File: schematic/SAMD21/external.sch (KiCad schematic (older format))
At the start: 19 parts, among them IC3 MCP2221-I_SL, J10 Conn_02x06_Odd_Even, J11 Conn_02x06_Odd_Even, J12 Conn_02x06_Odd_Even, J13 Conn_01x02, J14 Conn_02x05_Odd_Even, J15 Conn_01x08, J8 Conn_02x02_Odd_Even, J9 Conn_02x02_Odd_Even

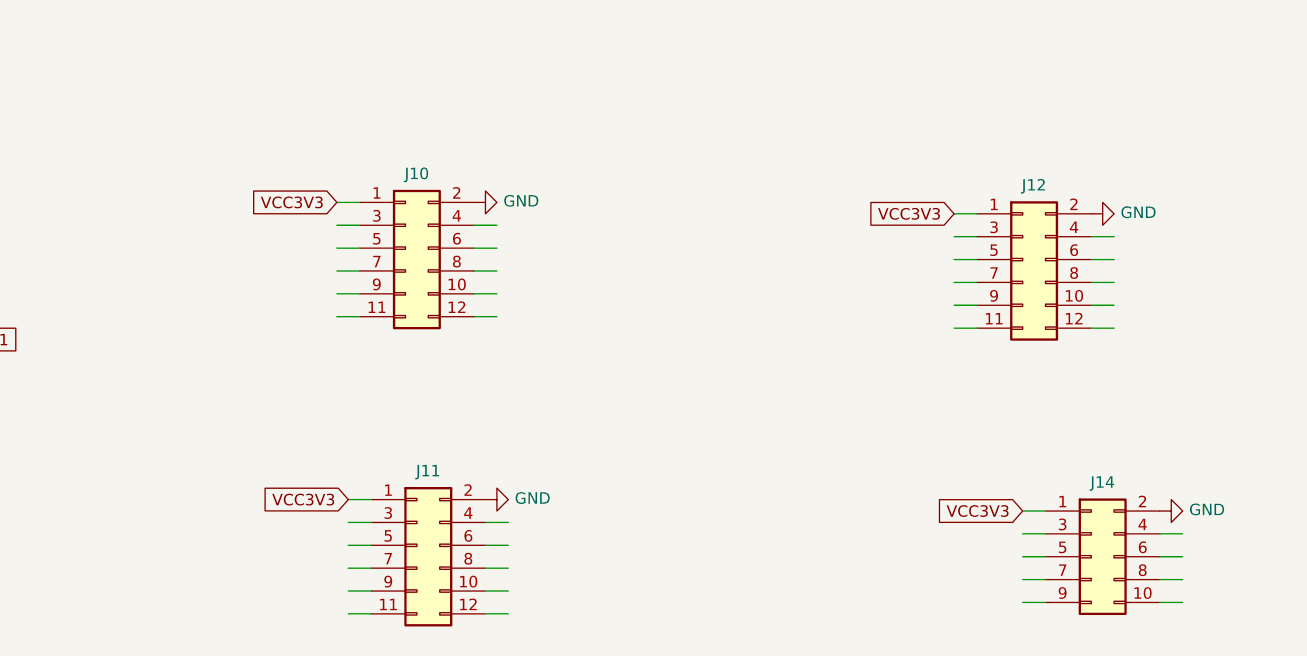
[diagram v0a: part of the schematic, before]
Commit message: Complete schematic
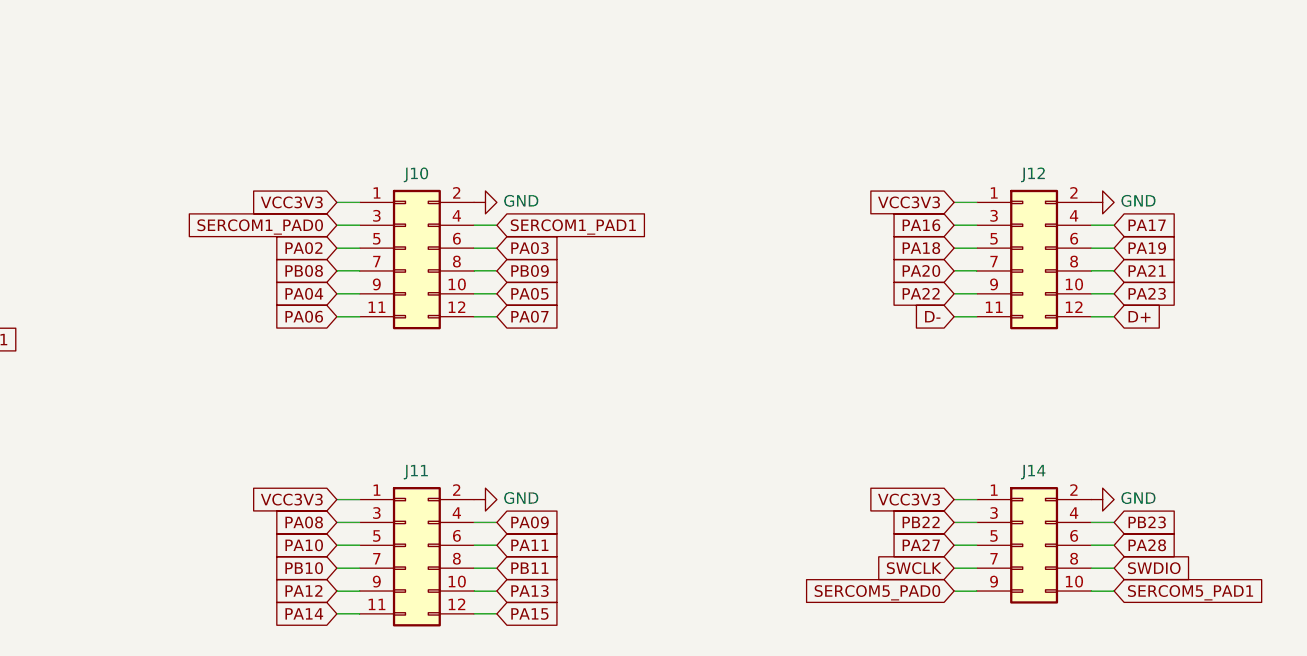
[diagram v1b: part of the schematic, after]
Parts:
- J10: footprint (none) -> Connector_PinHeader_2.54mm:PinHeader_2x06_P2.54mm_Vertical
- J12: footprint (none) -> Connector_PinHeader_2.54mm:PinHeader_2x06_P2.54mm_Vertical_SMD
- J14: footprint (none) -> Connector_PinHeader_2.54mm:PinHeader_2x05_P2.54mm_Vertical
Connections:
- net labels added: D+, D-, PA02, PA03, PA04, PA05, PA06, PA07, PA08, PA09, PA10, PA11, PA12, PA13, PA14, PA15, PA16, PA17, PA18, PA19, PA20, PA21, PA22, PA23, PA27, PA28, PB08, PB09, PB10, PB11, PB22, PB23
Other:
- moved on the sheet: J11, J12, J14
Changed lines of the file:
@@
 L Connector_Generic:Conn_02x06_Odd_Even J11
 U 1 1 61799C22
-P 4850 5800
-F 0 "J11" H 4900 6125 50  0000 C CNN
-F 1 "Conn_02x06_Odd_Even" H 4900 6126 50  0001 C CNN
-F 2 "Connector_PinHeader_2.54mm:PinHeader_2x06_P2.54mm_Vertical" H 4850 5800 50  0001 C CNN
-F 3 "~" H 4850 5800 50  0001 C CNN
-	1    4850 5800
-	1    0    0    -1
-$EndComp
-Text GLabel 7200 4350 0    50   Input ~ 0
-VCC3V3
-Text GLabel 4550 5600 0    50   Input ~ 0
-VCC3V3
-Text GLabel 7500 5650 0    50   Input ~ 0
+P 4800 5800
+F 0 "J11" H 4850 6125 50  0000 C CNN
+F 1 "Conn_02x06_Odd_Even" H 4850 6126 50  0001 C CNN
+F 2 "Connector_PinHeader_2.54mm:PinHeader_2x06_P2.54mm_Vertical" H 4800 5800 50  0001 C CNN
+F 3 "~" H 4800 5800 50  0001 C CNN
+	1    4800 5800
+	1    0    0    -1
+$EndComp
+Text GLabel 7200 4300 0    50   Input ~ 0
+VCC3V3
+Text GLabel 4500 5600 0    50   Input ~ 0
+VCC3V3
+Text GLabel 7200 5600 0    50   Input ~ 0
 VCC3V3
 $Comp
 L power:GND #PWR029
 U 1 1 617AC5C9
-P 7800 4350
-F 0 "#PWR029" H 7800 4100 50  0001 C CNN
-F 1 "GND" V 7805 4222 50  0000 R CNN
-F 2 "" H 7800 4350 50  0001 C CNN
-F 3 "" H 7800 4350 50  0001 C CNN
-	1    7800 4350
+P 7800 4300
+F 0 "#PWR029" H 7800 4050 50  0001 C CNN
+F 1 "GND" V 7805 4172 50  0000 R CNN
+F 2 "" H 7800 4300 50  0001 C CNN
+F 3 "" H 7800 4300 50  0001 C CNN
+	1    7800 4300
 	0    -1   -1   0
 $EndComp
@@
 L power:GND #PWR027
 U 1 1 617B03D0
-P 5150 5600
-F 0 "#PWR027" H 5150 5350 50  0001 C CNN
-F 1 "GND" V 5155 5472 50  0000 R CNN
-F 2 "" H 5150 5600 50  0001 C CNN
-F 3 "" H 5150 5600 50  0001 C CNN
-	1    5150 5600
+P 5100 5600
+F 0 "#PWR027" H 5100 5350 50  0001 C CNN
+F 1 "GND" V 5105 5472 50  0000 R CNN
+F 2 "" H 5100 5600 50  0001 C CNN
+F 3 "" H 5100 5600 50  0001 C CNN
+	1    5100 5600
 	0    -1   -1   0
 $EndComp
@@
 L power:GND #PWR030
 U 1 1 617B4203
-P 8100 5650
-F 0 "#PWR030" H 8100 5400 50  0001 C CNN
-F 1 "GND" V 8105 5522 50  0000 R CNN
-F 2 "" H 8100 5650 50  0001 C CNN
-F 3 "" H 8100 5650 50  0001 C CNN
-	1    8100 5650
+P 7800 5600
+F 0 "#PWR030" H 7800 5350 50  0001 C CNN
+F 1 "GND" V 7805 5472 50  0000 R CNN
+F 2 "" H 7800 5600 50  0001 C CNN
+F 3 "" H 7800 5600 50  0001 C CNN
+	1    7800 5600
 	0    -1   -1   0
 $EndComp
@@
 	5200 4400 5100 4400
 Wire Wire Line
-	7200 4350 7300 4350
-Wire Wire Line
-	7300 4450 7200 4450
-Wire Wire Line
-	7200 4550 7300 4550
-Wire Wire Line
-	7300 4650 7200 4650
-Wire Wire Line
-	7200 4750 7300 4750
-Wire Wire Line
-	7300 4850 7200 4850
-Wire Wire Line
-	7900 4850 7800 4850
-Wire Wire Line
-	7800 4750 7900 4750
-Wire Wire Line
-	7900 4650 7800 4650
-Wire Wire Line
-	7800 4550 7900 4550
-Wire Wire Line
-	7900 4450 7800 4450
-Wire Wire Line
-	4550 5600 4650 5600
-Wire Wire Line
-	4650 5700 4550 5700
-Wire Wire Line
-	4550 5800 4650 5800
-Wire Wire Line
-	4650 5900 4550 5900
-Wire Wire Line
-	4550 6000 4650 6000
-Wire Wire Line
-	4550 6100 4650 6100
-Wire Wire Line
-	5150 6100 5250 6100
-Wire Wire Line
-	5250 6000 5150 6000
-Wire Wire Line
-	5150 5900 5250 5900
-Wire Wire Line
-	5250 5800 5150 5800
-Wire Wire Line
-	5150 5700 5250 5700
-Wire Wire Line
-	7600 5650 7500 5650
-Wire Wire Line
-	7500 5750 7600 5750
-Wire Wire Line
-	8100 5850 8200 5850
-Wire Wire Line
-	8200 5950 8100 5950
-Wire Wire Line
-	8100 6050 8200 6050
-Wire Wire Line
-	7600 6050 7500 6050
-Wire Wire Line
-	7500 5950 7600 5950
-Wire Wire Line
-	8100 5750 8200 5750
+	7200 4300 7300 4300
+Wire Wire Line
+	7300 4400 7200 4400
+Wire Wire Line
+	7200 4500 7300 4500
+Wire Wire Line
+	7300 4600 7200 4600
+Wire Wire Line
+	7200 4700 7300 4700
+Wire Wire Line
+	7300 4800 7200 4800
+Wire Wire Line
+	7900 4800 7800 4800
+Wire Wire Line
+	7800 4700 7900 4700
+Wire Wire Line
+	7900 4600 7800 4600
+Wire Wire Line
+	7800 4500 7900 4500
+Wire Wire Line
+	7900 4400 7800 4400
+Wire Wire Line
+	4500 5600 4600 5600
+Wire Wire Line
+	4600 5700 4500 5700
+Wire Wire Line
+	4500 5800 4600 5800
+Wire Wire Line
+	4600 5900 4500 5900
+Wire Wire Line
+	4500 6000 4600 6000
+Wire Wire Line
+	4500 6100 4600 6100
+Wire Wire Line
+	5100 6100 5200 6100
+Wire Wire Line
+	5200 6000 5100 6000
+Wire Wire Line
+	5100 5900 5200 5900
+Wire Wire Line
+	5200 5800 5100 5800
+Wire Wire Line
+	5100 5700 5200 5700
+Wire Wire Line
+	7300 5600 7200 5600
+Wire Wire Line
+	7200 5700 7300 5700
+Wire Wire Line
+	7800 5800 7900 5800
+Wire Wire Line
+	7900 5900 7800 5900
+Wire Wire Line
+	7800 6000 7900 6000
+Wire Wire Line
+	7300 6000 7200 6000
+Wire Wire Line
+	7200 5900 7300 5900
+Wire Wire Line
+	7800 5700 7900 5700
 $Comp
 L Connector_Generic:Conn_01x08 J15
@@
 Program/Debug
 Wire Wire Line
-	7500 5850 7600 5850
+	7200 5800 7300 5800
 Text Notes 2900 2900 0    50   ~ 0
 SERCOM1
@@
 F 0 "J10" H 4850 4825 50  0000 C CNN
 F 1 "Conn_02x06_Odd_Even" H 4850 4826 50  0001 C CNN
-F 2 "" H 4800 4500 50  0001 C CNN
+F 2 "Connector_PinHeader_2.54mm:PinHeader_2x06_P2.54mm_Vertical" H 4800 4500 50  0001 C CNN
 F 3 "~" H 4800 4500 50  0001 C CNN
 	1    4800 4500
@@
 L Connector_Generic:Conn_02x06_Odd_Even J12
 U 1 1 619CB274
-P 7500 4550
-F 0 "J12" H 7550 4875 50  0000 C CNN
-F 1 "Conn_02x06_Odd_Even" H 7550 4876 50  0001 C CNN
-F 2 "" H 7500 4550 50  0001 C CNN
-F 3 "~" H 7500 4550 50  0001 C CNN
-	1    7500 4550
+P 7500 4500
+F 0 "J12" H 7550 4825 50  0000 C CNN
+F 1 "Conn_02x06_Odd_Even" H 7550 4826 50  0001 C CNN
+F 2 "Connector_PinHeader_2.54mm:PinHeader_2x06_P2.54mm_Vertical_SMD" H 7500 4500 50  0001 C CNN
+F 3 "~" H 7500 4500 50  0001 C CNN
+	1    7500 4500
 	1    0    0    -1
 $EndComp
@@
 L Connector_Generic:Conn_02x05_Odd_Even J14
 U 1 1 619D2D7D
-P 7800 5850
-F 0 "J14" H 7850 6175 50  0000 C CNN
-F 1 "Conn_02x05_Odd_Even" H 7850 6176 50  0001 C CNN
-F 2 "" H 7800 5850 50  0001 C CNN
-F 3 "~" H 7800 5850 50  0001 C CNN
-	1    7800 5850
-	1    0    0    -1
-$EndComp
+P 7500 5800
+F 0 "J14" H 7550 6125 50  0000 C CNN
+F 1 "Conn_02x05_Odd_Even" H 7550 6126 50  0001 C CNN
+F 2 "Connector_PinHeader_2.54mm:PinHeader_2x05_P2.54mm_Vertical" H 7500 5800 50  0001 C CNN
+F 3 "~" H 7500 5800 50  0001 C CNN
+	1    7500 5800
+	1    0    0    -1
+$EndComp
+Text GLabel 4500 4400 0    50   Input ~ 0
+SERCOM1_PAD0
+Text GLabel 5200 4400 2    50   Input ~ 0
+SERCOM1_PAD1
+Text GLabel 4500 4500 0    50   Input ~ 0
+PA02
+Text GLabel 5200 4500 2    50   Input ~ 0
+PA03
+Text GLabel 4500 4600 0    50   Input ~ 0
+PB08
+Text GLabel 5200 4600 2    50   Input ~ 0
+PB09
+Text GLabel 4500 4700 0    50   Input ~ 0
+PA04
+Text GLabel 5200 4700 2    50   Input ~ 0
+PA05
+Text GLabel 4500 4800 0    50   Input ~ 0
+PA06
+Text GLabel 5200 4800 2    50   Input ~ 0
+PA07
+Text GLabel 4500 5700 0    50   Input ~ 0
+PA08
+Text GLabel 5200 5700 2    50   Input ~ 0
+PA09
+Text GLabel 4500 5800 0    50   Input ~ 0
+PA10
+Text GLabel 5200 5800 2    50   Input ~ 0
+PA11
+Text GLabel 4500 5900 0    50   Input ~ 0
+PB10
+Text GLabel 5200 5900 2    50   Input ~ 0
+PB11
+Text GLabel 4500 6000 0    50   Input ~ 0
+PA12
+Text GLabel 5200 6000 2    50   Input ~ 0
+PA13
+Text GLabel 4500 6100 0    50   Input ~ 0
+PA14
+Text GLabel 5200 6100 2    50   Input ~ 0
+PA15
+Text GLabel 7200 4400 0    50   Input ~ 0
+PA16
+Text GLabel 7900 4400 2    50   Input ~ 0
+PA17
+Text GLabel 7200 4500 0    50   Input ~ 0
+PA18
+Text GLabel 7900 4500 2    50   Input ~ 0
+PA19
+Text GLabel 7200 4600 0    50   Input ~ 0
+PA20
+Text GLabel 7900 4600 2    50   Input ~ 0
+PA21
+Text GLabel 7200 4700 0    50   Input ~ 0
+PA22
+Text GLabel 7900 4700 2    50   Input ~ 0
+PA23
+Text GLabel 7200 4800 0    50   Input ~ 0
+D-
+Text GLabel 7900 4800 2    50   Input ~ 0
+D+
+Text GLabel 7200 5700 0    50   Input ~ 0
+PB22
+Text GLabel 7900 5700 2    50   Input ~ 0
+PB23
+Text GLabel 7200 5800 0    50   Input ~ 0
+PA27
+Text GLabel 7900 5800 2    50   Input ~ 0
+PA28
+Text GLabel 7200 5900 0    50   Input ~ 0
+SWCLK
+Text GLabel 7900 5900 2    50   Input ~ 0
+SWDIO
+Text GLabel 7200 6000 0    50   Input ~ 0
+SERCOM5_PAD0
+Text GLabel 7900 6000 2    50   Input ~ 0
+SERCOM5_PAD1
 $EndSCHEMATC
